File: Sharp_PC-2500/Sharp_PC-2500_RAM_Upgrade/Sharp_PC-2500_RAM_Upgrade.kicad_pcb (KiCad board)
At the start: 2 copper layers, 4 parts, among them J1 Conn_01x30, U1 74HCT04, U2 62256

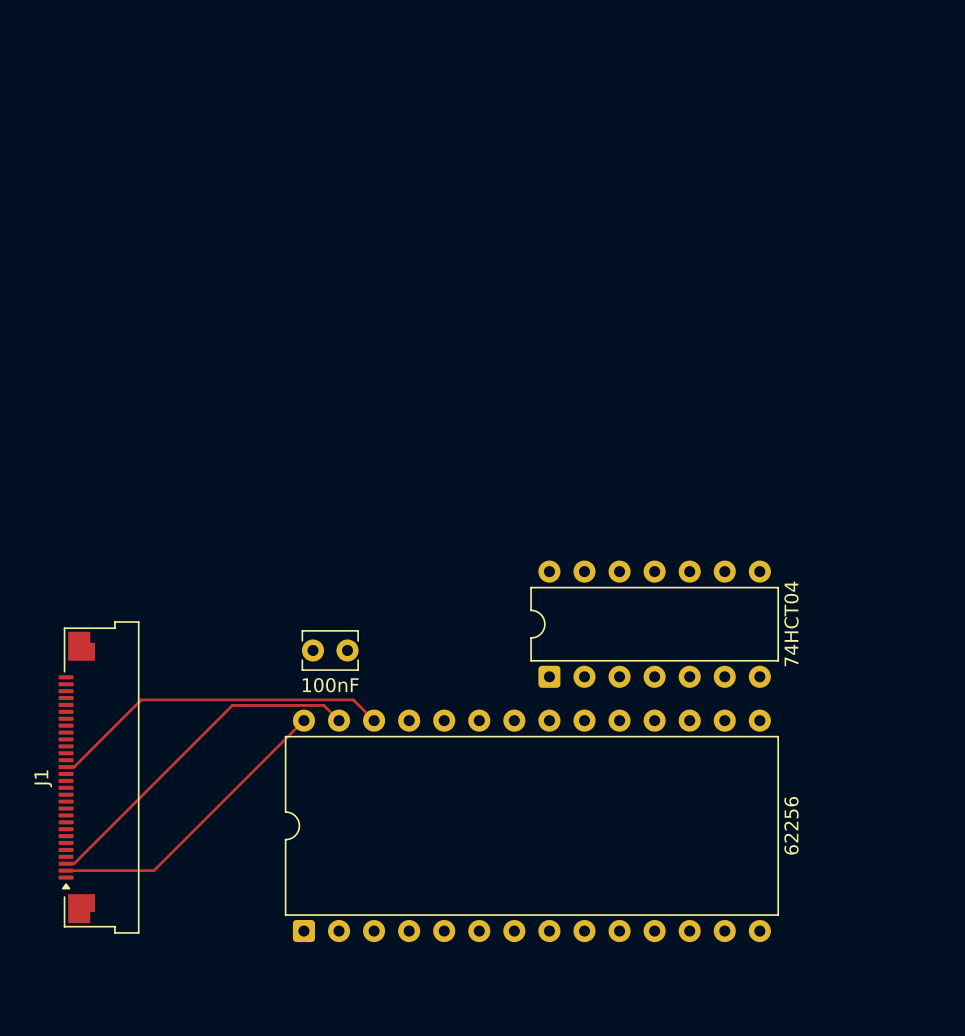
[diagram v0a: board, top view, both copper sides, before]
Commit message: Initial commit
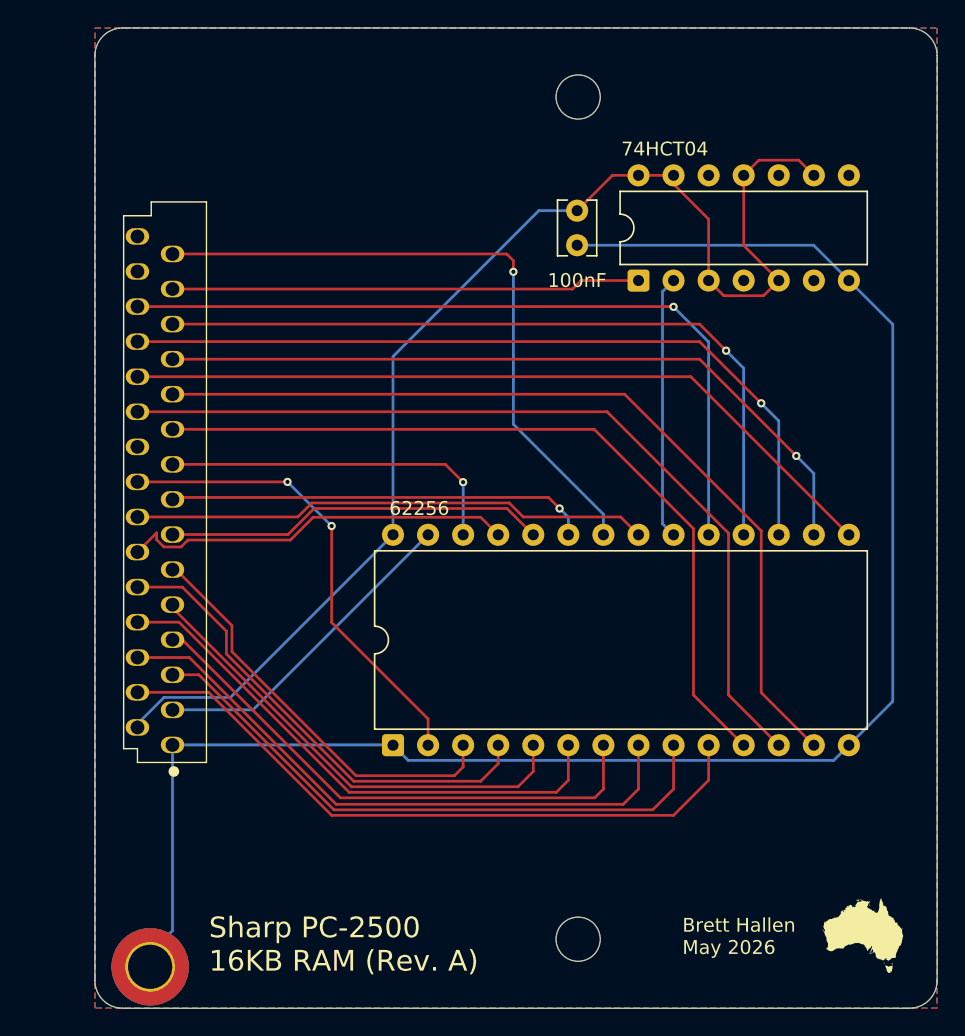
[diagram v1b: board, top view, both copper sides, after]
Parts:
- removed J1: Conn_01x30, Connector_FFC-FPC:Amphenol_F32Q-1A7x1-11030_1x30-1MP_P0.5mm_Horizontal
- added H1: MountingHole_Pad, MountingHole:MountingHole_3.2mm_M3_DIN965_Pad_TopBottom, F.Cu at (93.0, 108.0)
- added H2: MountingHole, MountingHole:MountingHole_3.2mm_M3, F.Cu at (124.0, 45.0)
- added H3: MountingHole, MountingHole:MountingHole_3.2mm_M3, F.Cu at (124.0, 106.0)
- added J2: FPC, Sharp_PC-2500:Sharp PC-2500 30-pin TFC Connector, F.Cu at (92.1, 55.1)
- moved C1 37.2 mm to (123.9, 53.2), turned to -90 degrees
- moved U1 29.4 mm to (128.4, 58.3)
- moved U2 14.9 mm to (110.6, 92.0)
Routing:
- net GND: track 0.00 -> 124.1 mm
- net VCC: track 21.7 -> 92.4 mm
- net /D2: track 0.00 -> 63.8 mm
- net /D1: track 0.00 -> 63.3 mm
- net /D0: track 0.00 -> 57.9 mm
- net /D5: track 0.00 -> 57.1 mm, vias 0 -> 1
- net /D7: track 0.00 -> 56.4 mm, vias 0 -> 1
- net /D3: track 0.00 -> 56.3 mm
- net /D6: track 0.00 -> 54.8 mm, vias 0 -> 1
- net /D4: track 0.00 -> 54.3 mm, vias 0 -> 1
- net /A0: track 0.00 -> 48.7 mm
- net /~{OE}: track 0.00 -> 47.4 mm, vias 0 -> 1
- net /A2: track 0.00 -> 44.3 mm
- net /A1: track 0.00 -> 44.1 mm
- net /A3: track 0.00 -> 39.4 mm
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- added copper zone on B.Cu, net GND
- added copper zone on F.Cu, net GND
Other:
- board outline added: 61 x 71 mm
- board text added: "Brett Hallen May 2026"
- board text added: "Sharp PC-2500 16KB RAM (Rev. A)"
